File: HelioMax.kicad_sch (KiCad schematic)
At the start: 72 parts, among them J1 Conn_01x01_Pin, J10 Conn_01x07, J11 Conn_01x07, J2 Conn_01x07, J3 Conn_01x07, J4 Conn_01x07, J5 Conn_01x07, J6 Conn_01x07, J7 Conn_01x07, J8 Conn_01x07, J9 Conn_01x07, SW0:10 SW0:3, SW0:11 SW0:2, SW0:12 SW0:1, SW0:7 SW0:6, SW0:8 SW0:5, SW0:9 SW0:4, SW1:10 SW1:3, SW1:11 SW1:2, SW1:12 SW1:1, SW1:13 SW1:0, SW1:9 SW1:4, SW2:10 SW2:3, SW2:11 SW2:2, SW2:12 SW2:1, SW2:13 SW2:0, SW2:7 SW2:6, SW2:8 SW2:5, SW2:9 SW2:4, SW3:10 SW3:3, SW3:11 SW3:2, SW3:12 SW3:1, SW3:13 SW3:0, SW3:8 SW3:5, SW3:9 SW3:4, SW4:10 SW4:3, SW4:11 SW4:2, SW4:12 SW4:1, SW4:13 SW4:0, SW4:7 SW4:6, SW4:8 SW4:5, SW4:9 SW4:4, SW5:10 SW5:3, SW5:11 SW5:2, SW5:12 SW5:1, SW5:13 SW5:0, SW5:7 SW5:6, SW5:8 SW5:5, SW5:9 SW5:4, SW6:10 SW6:3, SW6:11 SW6:2, SW6:12 SW6:1, SW6:13 SW6:0, SW6:7 SW6:6, SW6:8 SW6:5, SW6:9 SW6:4

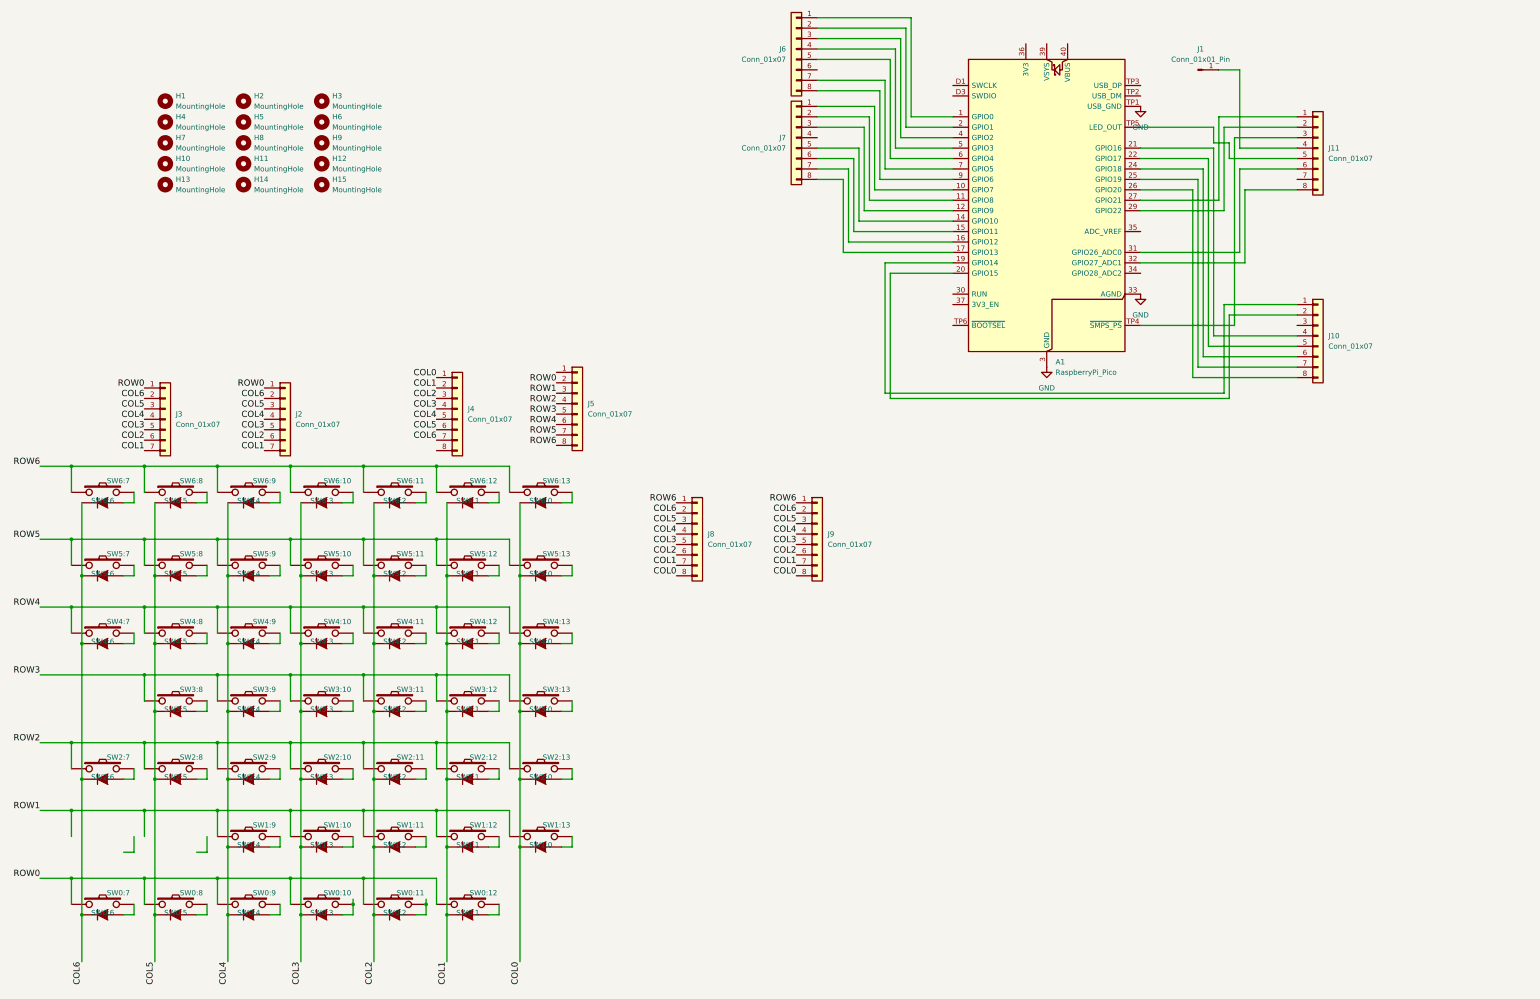
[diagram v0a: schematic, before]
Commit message: Added donations (as if anybody will do that)
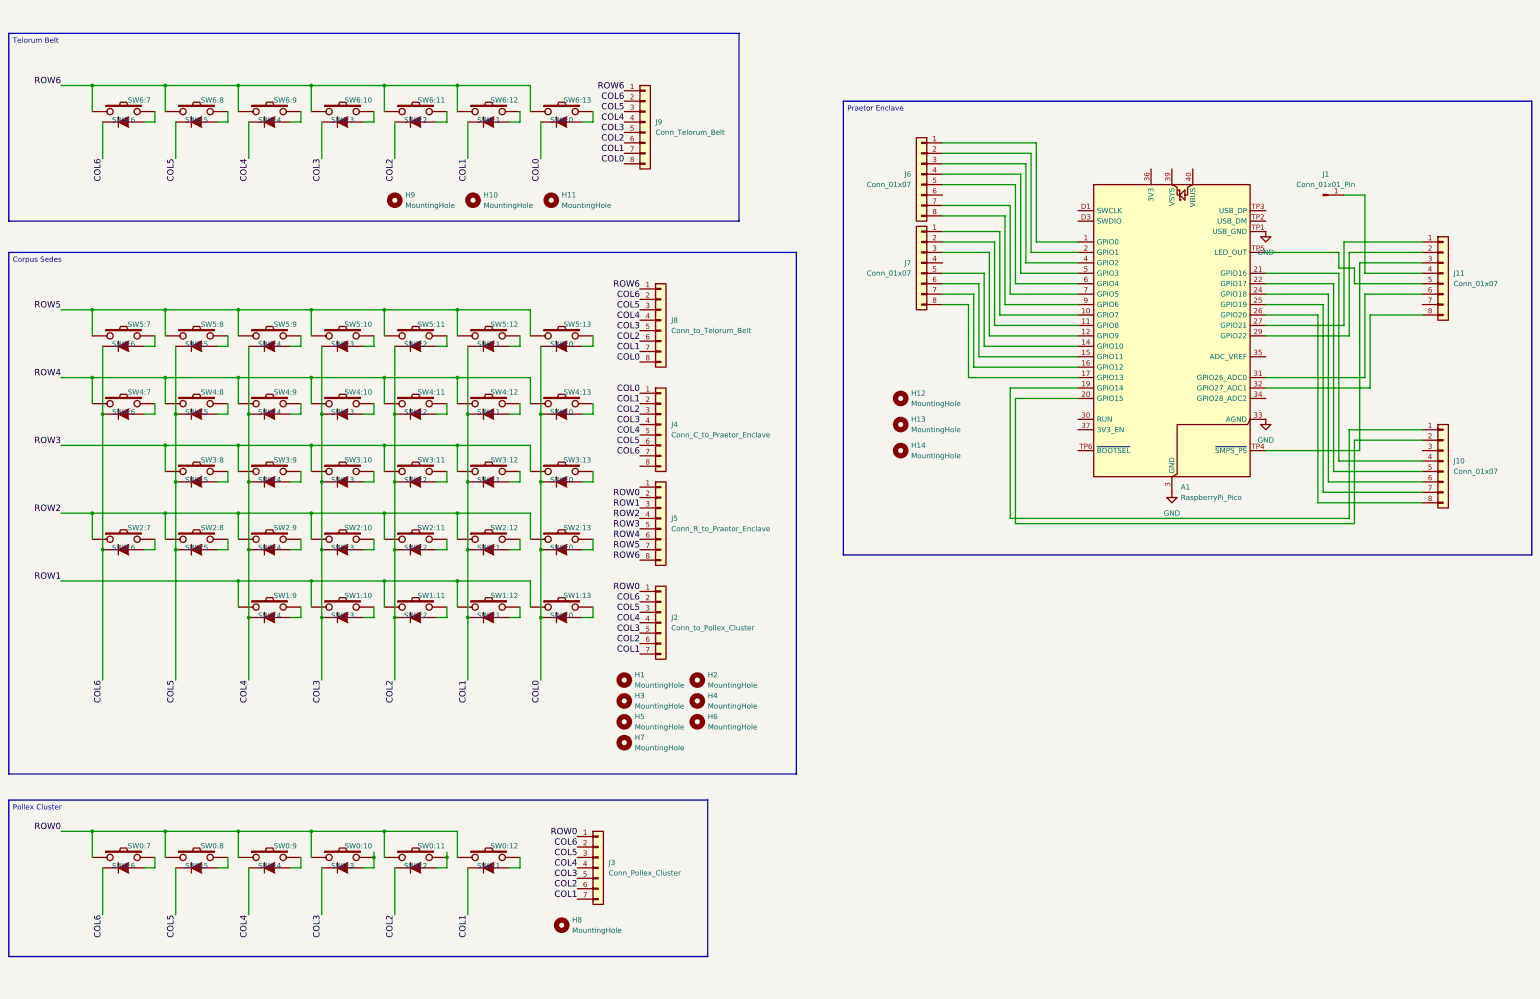
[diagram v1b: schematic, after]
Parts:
- removed H15: MountingHole, MountingHole:MountingHole_3.2mm_M3, symbol Mechanical:MountingHole
- J2: value Conn_01x07 -> Conn_to_Pollex_Cluster
- J3: value Conn_01x07 -> Conn_Pollex_Cluster
- J4: value Conn_01x07 -> Conn_C_to_Praetor_Enclave
- J5: value Conn_01x07 -> Conn_R_to_Praetor_Enclave
- J8: value Conn_01x07 -> Conn_to_Telorum_Belt
- J9: value Conn_01x07 -> Conn_Telorum_Belt
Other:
- moved on the sheet: A1, H1, H10, H11, H12, H13, H14, H2, H3, H4, H5, H6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
